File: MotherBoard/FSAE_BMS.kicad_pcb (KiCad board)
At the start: 4 copper layers, 110 x 115 mm, 223 parts, among them IC501 BQ79600PWRQ1, J201 Conn_ARM_SWD_TagConnect_TC2030, J202 DM3AT-SF-PEJM5_40_, J301 1376357-3, J302 Conn_01x04_Pin, J303 430450200, J304 430450200, Q701 Q_NPN_BEC, Q702 Q_NPN_BEC, Q703 Q_NPN_BEC, Q704 Q_NMOS_GDS, Q705 Q_NMOS_GDS, Q706 Q_NMOS_GDS, Q707 Q_NPN_BEC, Q708 Q_NMOS_GDS, U201 STM32F205RBTx, U401 LMR51430, U402 LMR51430, U601 PTCAN1462DRQ1, U602 PTCAN1462DRQ1, Y201 16 Mhz

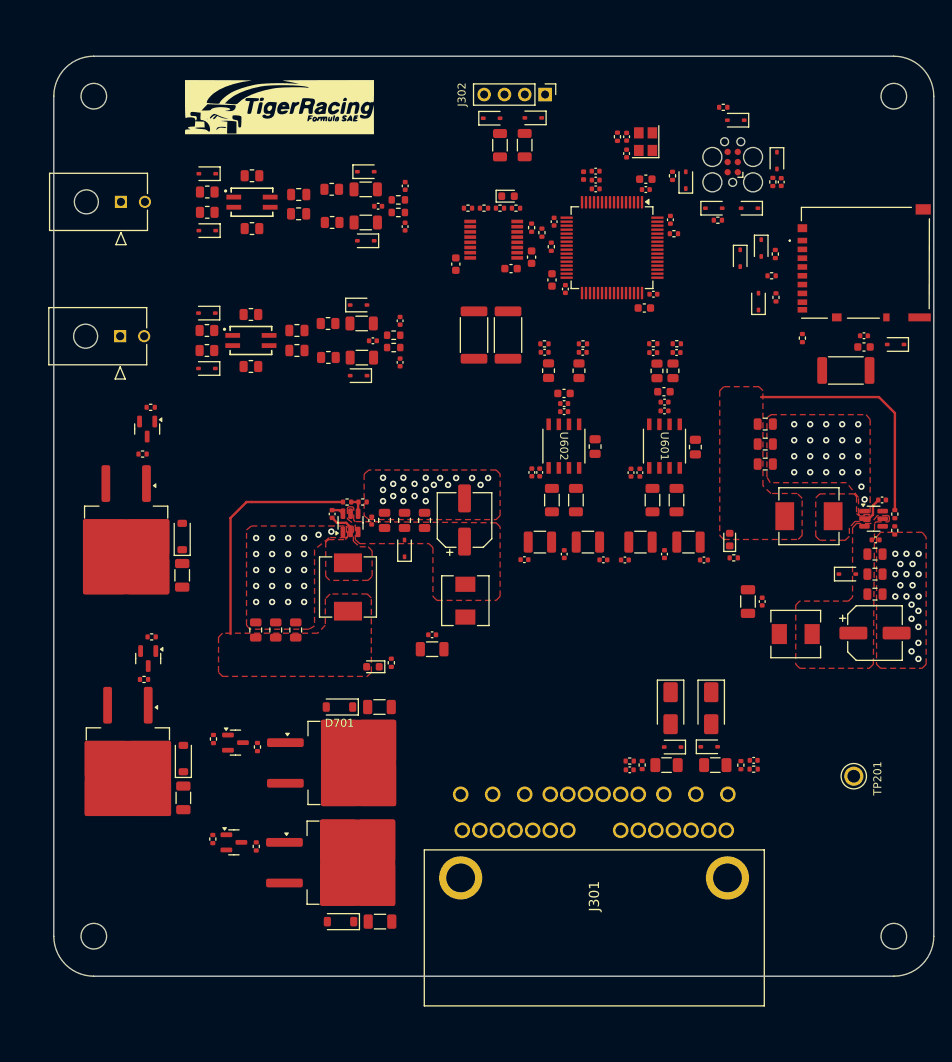
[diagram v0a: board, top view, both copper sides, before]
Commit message: Finished motherboard. Need to review BOM
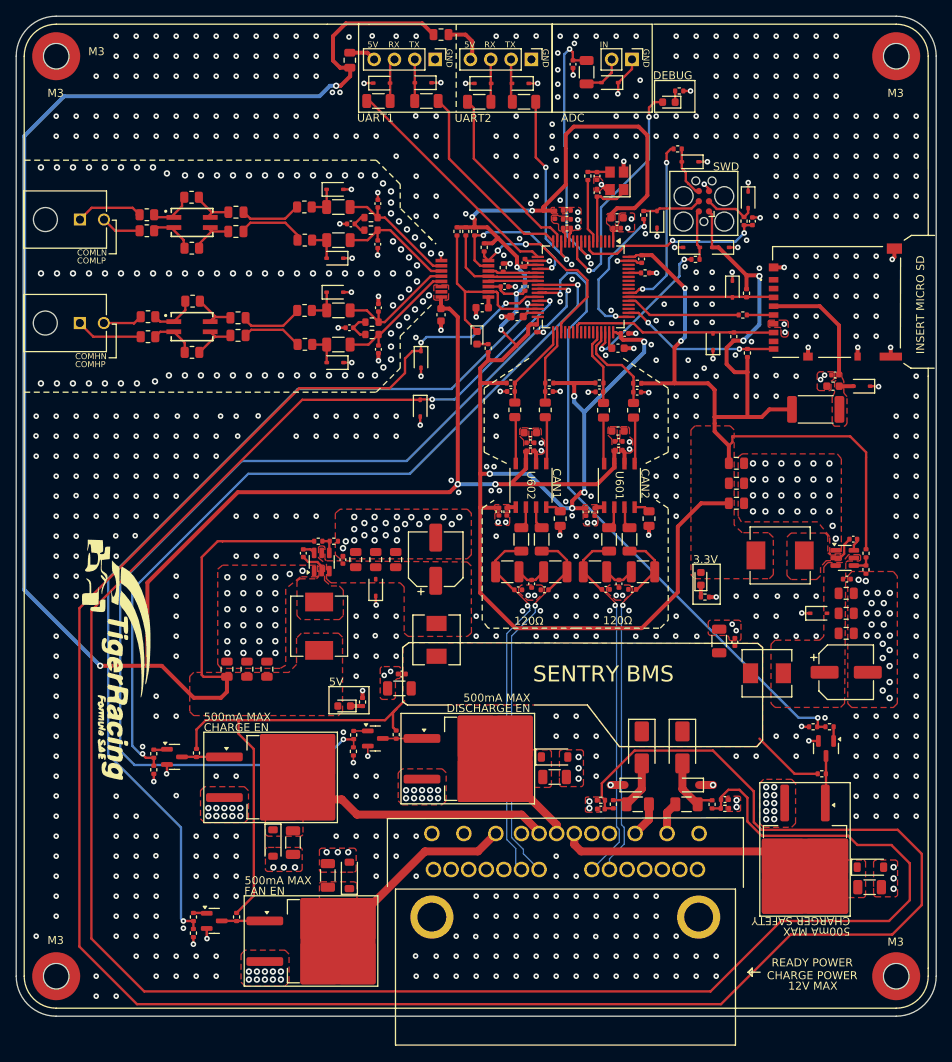
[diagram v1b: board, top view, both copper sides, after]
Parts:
- removed the D208 at (180.8, 55.2)
- removed the D304 at (114.2, 44.7)
- removed D306: D_TVS, Diode_SMD:D_SOD-323
- removed the J303 at (103.3, 65.0)
- removed the R402 at (147.5, 64.9)
- removed the R403 at (151.8, 64.9)
- removed TP201: TestPoint, TestPoint:TP_5012
- added C301: 1u, Capacitor_SMD:C_0402_1005Metric, F.Cu at (159.9, 31.0)
- added D202: GREEN, LED_SMD:LED_0603_1608Metric, F.Cu at (171.9, 35.7)
- added D301: D_TVS, Diode_SMD:D_SOD-323, F.Cu at (148.6, 33.4)
- added D401: D_Zener, Diode_SMD:D_SOD-323, F.Cu at (140.9, 67.9)
- added D402: D_Zener, Diode_SMD:D_SOD-323, F.Cu at (140.8, 74.0)
- added F301: Fuse, Fuse:Fuse_0805_2012Metric, F.Cu at (143.4, 27.3)
- added F302: Fuse, Fuse:Fuse_0805_2012Metric, F.Cu at (132.0, 30.5)
- added J301: Conn_01x04_Pin, Connector_PinHeader_2.54mm:PinHeader_1x04_P2.54mm_Vertical, F.Cu at (154.7, 30.4)
- added J304: 430450200, molex_comm:CON_430450200_MOL, F.Cu at (98.3, 63.4)
- added J306: Conn_01x02_Pin, Connector_PinHeader_2.54mm:PinHeader_1x02_P2.54mm_Vertical, F.Cu at (167.3, 30.4)
- added R201: 1k, Resistor_SMD:R_0402_1005Metric, F.Cu at (173.2, 34.3)
- added R301: 22R, Resistor_SMD:R_1206_3216Metric, F.Cu at (153.8, 35.7)
- added R302: 22R, Resistor_SMD:R_1206_3216Metric, F.Cu at (148.2, 35.7)
- added R305: 2.2k, Resistor_SMD:R_1206_3216Metric, F.Cu at (161.6, 32.0)
- added R701: 10k, Resistor_SMD:R_0402_1005Metric, F.Cu at (107.5, 119.2)
- added R702: 10k, Resistor_SMD:R_0402_1005Metric, F.Cu at (132.4, 116.9)
- added R703: 10k, Resistor_SMD:R_0402_1005Metric, F.Cu at (189.9, 113.8)
- added R710: 10k, Resistor_SMD:R_0402_1005Metric, F.Cu at (112.5, 139.6)
- C508: footprint Capacitor_SMD:C_0603_1608Metric -> Capacitor_SMD:C_0402_1005Metric
- moved H104 104.8 mm to (95.3, 145.0)
- moved H103 100.4 mm to (200.3, 145.0)
- moved D703 95.4 mm to (197.1, 131.4), turned to 0 degrees
- moved C703 94.4 mm to (197.0, 133.9), turned to 0 degrees
- moved R709 93.8 mm to (191.0, 119.7)
- moved R706 93.8 mm to (192.0, 113.8)
- moved Q703 93.8 mm to (191.5, 116.5)
- moved Q706 93.8 mm to (188.9, 131.0)
- moved G*** 72.0 mm to (102.8, 105.4), turned to -90 degrees
- moved D305 58.0 mm to (164.5, 33.3)
- moved D303 53.0 mm to (153.3, 33.4)
- moved C702 46.5 mm to (157.6, 120.1), turned to 0 degrees
- moved D702 46.4 mm to (157.6, 117.6), turned to 0 degrees
- moved Q705 44.4 mm to (148.7, 117.8), turned to 0 degrees
- moved R708 32.3 mm to (137.8, 114.8), turned to -90 degrees
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- renumbered D202 to D203, D203 to D204, D204 to D205, D205 to D206, D206 to D207, D207 to D208, D301 to D302, D302 to D304, J301 to J303, J304 to J305, R201 to R202, R202 to R203, R203 to R204, R204 to R205, R205 to R206, R206 to R207, R207 to R208, R208 to R209, R209 to R210, R210 to R211, R211 to R212, R301 to R303, R302 to R304, R404 to R402, R405 to R403, R406 to R404, R407 to R405, R408 to R406, R409 to R407, R410 to R408, R411 to R409, R412 to R410, R701 to R704, R702 to R705, R703 to R706, R704 to R707, R705 to R708, R706 to R709, R707 to R711, R708 to R712
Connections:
- C401 pad 1: /PSU/READY_PWR_LV -> READY_PWR_LV_ISO
- C402 pad 1: /PSU/CHARGE_PWR_LV -> CHARGE_PWR_LV_ISO
- C505 pad 2: /BQ79600/COMLP -> /BQ79600/COMLN
- C506 pad 1: /BQ79600/COMLN -> /BQ79600/COMLP
- D303 pad 2: ISO_COMHP -> Net-(D303-A2)
- D305 pad 2: ISO_COMHN -> Net-(D305-A2)
- J302 pad 1: unconnected-(J302-Pin_1-Pad1) -> GND
- J302 pad 4: GND -> Net-(J302-Pin_4)
- R401 pad 1: /PSU/READY_PWR_LV -> READY_PWR_LV_ISO
- R402 pad 2: /PSU/READY_PWR_LV -> READY_PWR_LV_ISO
- R403 pad 2: /PSU/CHARGE_PWR_LV -> CHARGE_PWR_LV_ISO
- R404 pad 1: /PSU/CHARGE_PWR_LV -> CHARGE_PWR_LV_ISO
- R504 pad 1: /BQ79600/COMLP -> /BQ79600/COMLN
- R505 pad 2: /BQ79600/COMLN -> /BQ79600/COMLP
- R512 pad 1: /BQ79600/COMLP -> /BQ79600/COMLN
- R513 pad 1: /BQ79600/COMLN -> /BQ79600/COMLP
- R526 pad 2: ISO_COMLP -> ISO_COMLN
- R527 pad 2: ISO_COMLN -> ISO_COMLP
- R707 pad 1: +12V -> VBUS
- R708 pad 1: +12V -> VBUS
- R709 pad 1: +12V -> VBUS
- R712 pad 1: +12V -> VBUS
- U201 pad 10: unconnected-(U201-PC2-Pad10) -> /MCU/TEST_LED
- U201 pad 14: unconnected-(U201-PA0-Pad14) -> UART4_TX
- U201 pad 15: unconnected-(U201-PA1-Pad15) -> UART4_RX
- U201 pad 2: /MCU/SDIO_DET -> unconnected-(U201-PC13-Pad2)
- U201 pad 9: unconnected-(U201-PC1-Pad9) -> ADC_IN
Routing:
- net +3V3: track 29.6 -> 350.2 mm, vias 0 -> 14
- net CHARGE_PWR_LV_ISO: track 0.00 -> 290.9 mm, vias 0 -> 2
- net +5V: track 29.4 -> 293.7 mm, vias 0 -> 4
- net READY_PWR_LV_ISO: track 0.00 -> 262.5 mm, vias 0 -> 2
- net DISCHARGE_EN_LV: track 0.00 -> 129.4 mm, vias 0 -> 2
- net FAN_EN_LV: track 0.00 -> 117.7 mm, vias 0 -> 2
- net CHARGE_EN_LV: track 0.00 -> 101.9 mm, vias 0 -> 2
- net GND: track 0.00 -> 86.6 mm, vias 84 -> 993
- net CHARGE_SAFE_LV: track 0.00 -> 81.9 mm, vias 0 -> 2
- net VBUS: track 0.00 -> 67.8 mm
- net ISO_CAN2+: track 0.00 -> 46.8 mm, vias 0 -> 1
- net ISO_CAN1-: track 0.00 -> 46.4 mm, vias 0 -> 1
- net ISO_CAN2-: track 0.00 -> 46.3 mm, vias 0 -> 1
- net ISO_CAN1+: track 0.00 -> 45.9 mm, vias 0 -> 1
- net ADC_IN: track 0.00 -> 33.1 mm, vias 0 -> 2
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- added copper zone on F.Cu, net +3.3VP
- added copper zone on F.Cu, net CHARGE_EN_HV
- added copper zone on F.Cu, net CHARGE_SAFE_HV
- added copper zone on F.Cu, net DISCHARGE_EN_HV
- added copper zone on F.Cu, net FAN_EN_HV
- added copper zone on F.Cu, net VBUS
- added copper zone on F.Cu, net VDDA
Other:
- board size 110 x 115 mm -> 115 x 125 mm
- board text added: "120Ω"
- board text added: "12V MAX"
- board text added: "3.3V"
- board text added: "500mA MAX"
- board text added: "5V"
- board text added: "ADC"
- board text added: "CAN1"
- board text added: "CAN2"
- board text added: "CHARGE EN"
- board text added: "CHARGER SAFETY"
- board text added: "COMHN"
- board text added: "COMHP"
- board text added: "COMLN"
- board text added: "COMLP"
- board text added: "DEBUG"
- board text added: "DISCHARGE EN"
- board text added: "FAN EN"
- board text added: "GND"
- board text added: "IN"
- board text added: "INSERT MICRO SD"
- board text added: "M3"
- board text added: "READY POWER CHARGE POWER"
- board text added: "RX"
- board text added: "SENTRY BMS"
- board text added: "SWD"
- board text added: "TX"
- board text added: "UART1"
- board text added: "UART2"
- board text added: "https://github.com/JacobParent7/FSAE_LSU_BMS"
